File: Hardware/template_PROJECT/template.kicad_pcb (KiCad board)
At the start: 4 copper layers, 25 x 25 mm, 7 parts

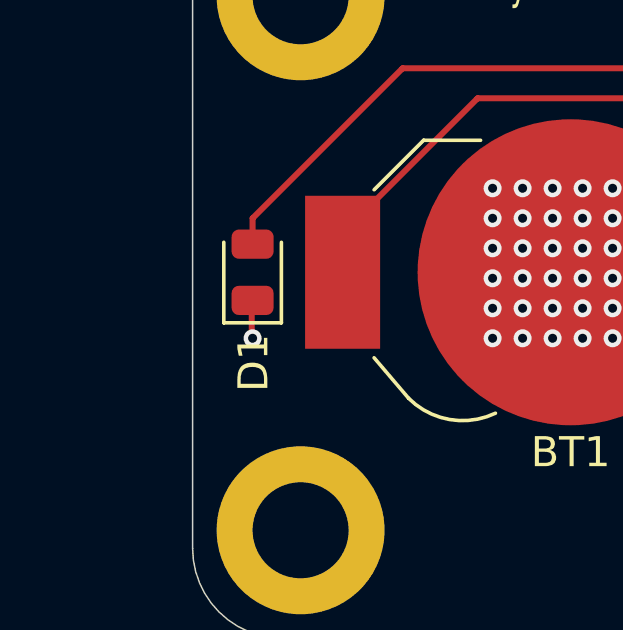
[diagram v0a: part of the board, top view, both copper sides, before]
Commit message: make it fail
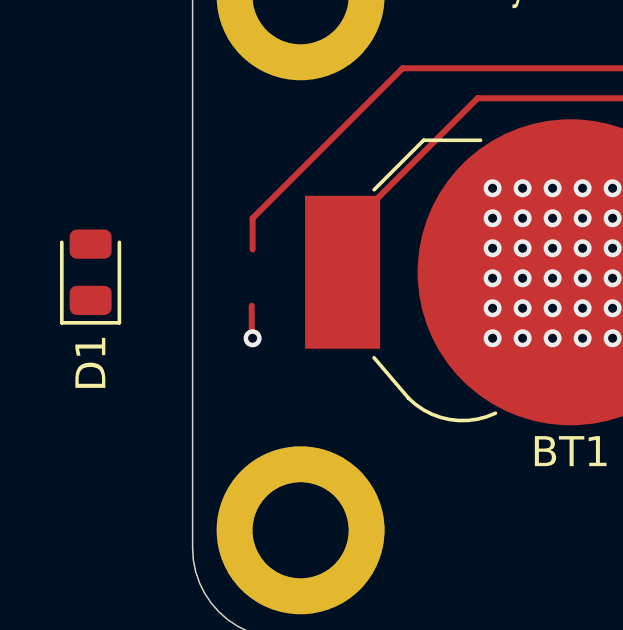
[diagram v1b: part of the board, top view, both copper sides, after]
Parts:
- moved D1 5.40 mm to (124.8, 100.4)
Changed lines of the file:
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@@
 	(footprint "LED_SMD:LED_0805_2012Metric"
 		(layer "F.Cu")
-		(at 130.2 100.4 90)
+		(at 124.8 100.4 90)
 		(descr "LED SMD 0805 (2012 Metric), square (rectangular) end terminal, IPC_7351 nominal, (Body size source: https://docs.google.com/spreadsheets/d/1BsfQQcO9C6DZCsRaXUlFlo91Tg2WpOkGARC1WS5S8t0/edit?usp=sharing), generated with kicad-footprint-generator")
 		(tags "LED")

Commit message: shouldnt fail now
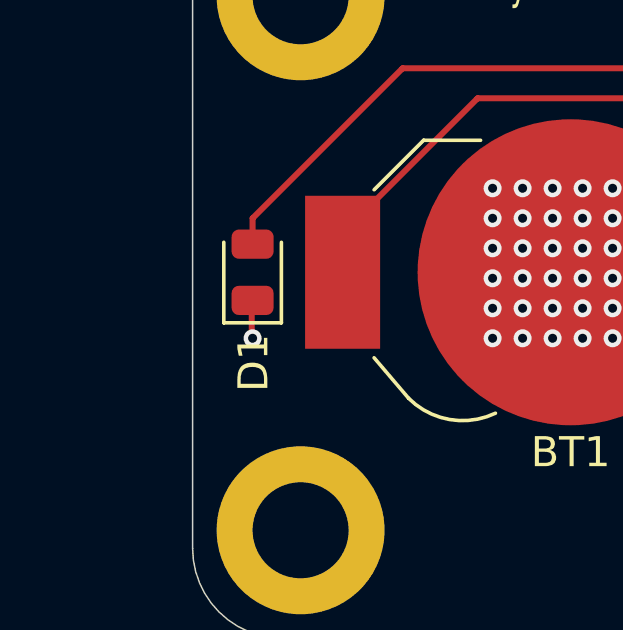
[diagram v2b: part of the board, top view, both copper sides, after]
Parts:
- moved D1 5.40 mm to (130.2, 100.4)
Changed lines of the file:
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@@
 	(footprint "LED_SMD:LED_0805_2012Metric"
 		(layer "F.Cu")
-		(at 124.8 100.4 90)
+		(at 130.2 100.4 90)
 		(descr "LED SMD 0805 (2012 Metric), square (rectangular) end terminal, IPC_7351 nominal, (Body size source: https://docs.google.com/spreadsheets/d/1BsfQQcO9C6DZCsRaXUlFlo91Tg2WpOkGARC1WS5S8t0/edit?usp=sharing), generated with kicad-footprint-generator")
 		(tags "LED")
